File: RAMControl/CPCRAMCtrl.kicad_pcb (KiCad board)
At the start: 2 copper layers, 99.1 x 52.9 mm, 31 parts, among them IC112 74LS32, IC118 AMG40031, IC192 74LS32, J1 Conn_01x10_Female, J2 Conn_01x16_Female, U114 74LS373, U115 74LS244, U191 74LS04, U193 74LS08, U194 74LS173, U195 74LS74

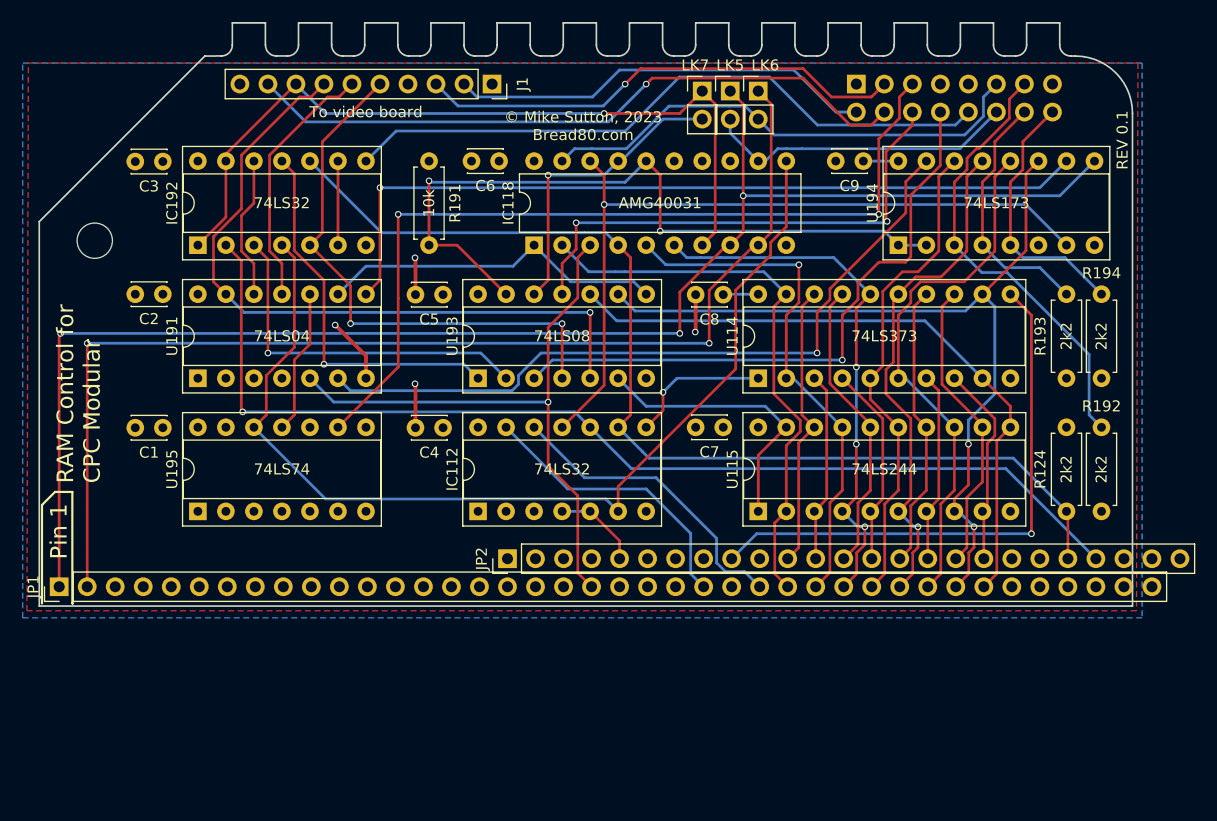
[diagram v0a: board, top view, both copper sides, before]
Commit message: Long overdue update...
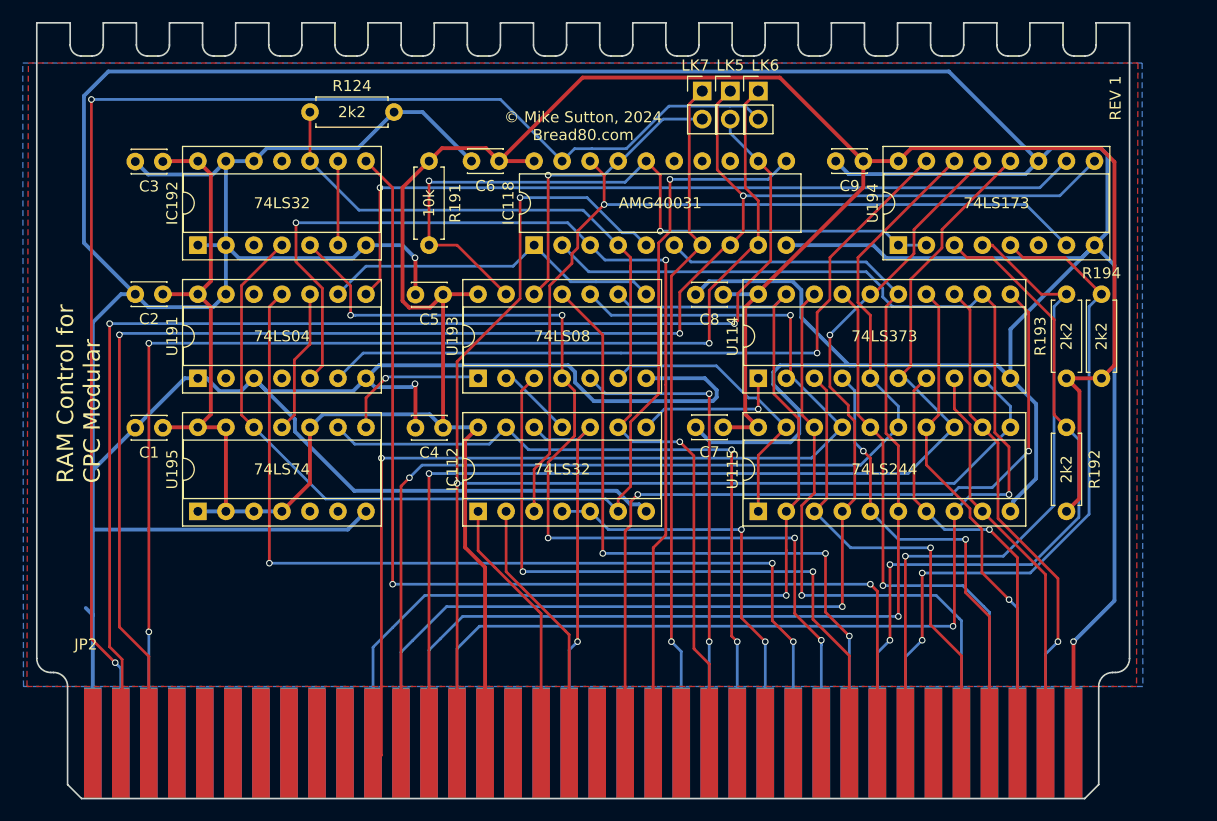
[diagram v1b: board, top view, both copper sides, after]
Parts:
- removed ?: , Mounting_Holes:MountingHole_3.2mm_M3
- removed J1: Conn_01x10_Female, Connector_PinSocket_2.54mm:PinSocket_1x10_P2.54mm_Vertical
- removed J2: Conn_01x16_Female, Connector_PinHeader_2.54mm:PinHeader_2x08_P2.54mm_Vertical
- JP1: value RC2014Bus -> CPCM_VideoRAM_EdgeBottom; footprint Connector_PinHeader_2.54mm:PinHeader_1x40_P2.54mm_Vertical -> CPCModular:Edge36_2.54PS; moved to B.Cu
- JP2: value RC2014ExtendedBus -> CPCM_VideoRAM_EdgeTop; footprint Connector_PinHeader_2.54mm:PinHeader_1x25_P2.54mm_Vertical -> CPCModular:Edge36_2.54PS
- moved R124 77.5 mm to (178.4, 108.6), turned to 0 degrees
- moved JP2 41.9 mm to (158.8, 167.6)
- moved JP1 12.7 mm to (158.8, 163.9), turned to 270 degrees
- moved R192 3.18 mm to (247.0, 144.8)
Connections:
- net ~CPU_ADDRx renamed /CRTC_ADDR_MULTI/~BUF_CPU_AD
- IC112 pad 1: GND -> /CRTC_ADDR_MULTI/~IORQ
- IC112 pad 12: /CRTC_ADDR_MULTI/~IORQ -> /~RAMRD
- IC112 pad 13: /CRTC_ADDR_MULTI/~WR -> /CRTC_ADDR_MULTI/~XCPU_AD
- IC112 pad 2: GND -> /CRTC_ADDR_MULTI/~WR
- IC118 pad 12: /CRTC_ADDR_MULTI/RAMA15 -> /CRTC_ADDR_MULTI/AOUT15
- IC118 pad 18: Net-(IC112-Pad11) -> Net-(IC112-Pad3)
- IC118 pad 19: /CRTC_ADDR_MULTI/RAMA14 -> /CRTC_ADDR_MULTI/AOUT14
- IC192 pad 1: /CRTC_ADDR_MULTI/~CAS -> GND
- IC192 pad 12: Net-(IC192-Pad12) -> GND
- IC192 pad 13: /CRTC_ADDR_MULTI/~CAS -> GND
- IC192 pad 2: /~RAMRD -> GND
- JP1 pad 1: A15 -> GND
- JP1 pad 11: Net-(JP1-Pad11) -> D6
- JP1 pad 12: Net-(JP1-Pad12) -> D4
- JP1 pad 13: Net-(JP1-Pad13) -> D2
- JP1 pad 14: Net-(JP1-Pad14) -> D0
- JP1 pad 17: GND -> Net-(JP1-Pad17)
- JP1 pad 18: +5V -> /~RAMRD
- JP1 pad 2: A14 -> /CRTC_ADDR_MULTI/AOUT14
- JP1 pad 20: /CRTC_ADDR_MULTI/~RESET -> Net-(JP1-Pad20)
- JP1 pad 22: Net-(JP1-Pad22) -> /CRTC_ADDR_MULTI/~CAS
- JP1 pad 23: Net-(JP1-Pad23) -> /CRTC_ADDR_MULTI/~244EN
- JP1 pad 24: /CRTC_ADDR_MULTI/~WR -> /CRTC_ADDR_MULTI/~XCPU_AD
- JP1 pad 25: Net-(JP1-Pad25) -> /~CPU_ADDR
- JP1 pad 26: /CRTC_ADDR_MULTI/~IORQ -> /CRTC_ADDR_MULTI/~RAS
- JP1 pad 27: D0 -> /CRTC_ADDR_MULTI/~MWE
- JP1 pad 28: D1 -> /CRTC_ADDR_MULTI/~RAMCS
- JP1 pad 29: D2 -> /CRTC_ADDR_MULTI/RAMA18
- JP1 pad 3: Net-(JP1-Pad3) -> A14
- JP1 pad 30: D3 -> /CRTC_ADDR_MULTI/RAMA16
- JP1 pad 31: D4 -> Net-(JP1-Pad31)
- JP1 pad 32: D5 -> RD6
- JP1 pad 33: D6 -> RD4
- JP1 pad 34: D7 -> RD2
- JP1 pad 35: Net-(JP1-Pad35) -> RD0
- JP2 pad 1: GND -> Net-(JP2-Pad1)
- JP2 pad 11: RAMD0 -> D7
- JP2 pad 12: RAMD1 -> D5
- JP2 pad 13: RAMD2 -> D3
- JP2 pad 14: RAMD3 -> D1
- JP2 pad 15: RAMD4 -> +5V
- JP2 pad 16: RAMD5 -> Net-(JP2-Pad16)
- JP2 pad 17: RAMD6 -> /CRTC_ADDR_MULTI/~IORQ
- JP2 pad 18: RAMD7 -> /CRTC_ADDR_MULTI/~WR
- JP2 pad 2: +5V -> /CRTC_ADDR_MULTI/AOUT15
- JP2 pad 20: Net-(JP2-Pad20) -> /READY
- JP2 pad 21: /RAMDIS -> /CRTC_ADDR_MULTI/~RESET
- JP2 pad 22: /~RAMRD -> Net-(JP2-Pad22)
- JP2 pad 23: Net-(JP2-Pad23) -> /RAMDIS
- JP2 pad 25: (no net) -> Net-(JP2-Pad25)
- JP2 pad 3: Net-(JP2-Pad3) -> A15
- JP2 pad 5: /~CPU_ADDR -> Net-(JP2-Pad5)
- JP2 pad 9: /READY -> Net-(JP2-Pad9)
- LK5 pad 2: /CRTC_ADDR_MULTI/RAMA15 -> /CRTC_ADDR_MULTI/AOUT15
- LK6 pad 2: /CRTC_ADDR_MULTI/RAMA14 -> /CRTC_ADDR_MULTI/AOUT14
- R192 pad 2: /CRTC_ADDR_MULTI/RAMA16 -> /CRTC_ADDR_MULTI/RAMA18
- R194 pad 2: /CRTC_ADDR_MULTI/RAMA18 -> /CRTC_ADDR_MULTI/RAMA16
- U114 pad 12: D6 -> D0
- U114 pad 13: RAMD6 -> RD0
- U114 pad 14: RAMD4 -> RD2
- U114 pad 15: D4 -> D2
- U114 pad 16: D2 -> D4
- U114 pad 17: RAMD2 -> RD4
- U114 pad 18: RAMD0 -> RD6
- U114 pad 19: D0 -> D6
- U114 pad 2: D1 -> D7
- U114 pad 3: RAMD1 -> RD7
- U114 pad 4: RAMD3 -> RD5
- U114 pad 5: D3 -> D5
- U114 pad 6: D5 -> D3
- U114 pad 7: RAMD5 -> RD3
- U114 pad 8: RAMD7 -> RD1
- U114 pad 9: D7 -> D1
- U115 pad 11: D7 -> D1
- U115 pad 12: RAMD6 -> RD0
- U115 pad 13: D5 -> D3
- U115 pad 14: RAMD4 -> RD2
- U115 pad 15: D3 -> D5
- U115 pad 16: RAMD2 -> RD4
- U115 pad 17: D1 -> D7
- U115 pad 18: RAMD0 -> RD6
- U115 pad 2: D0 -> D6
- U115 pad 3: RAMD1 -> RD7
- U115 pad 4: D2 -> D4
- U115 pad 5: RAMD3 -> RD5
- U115 pad 6: D4 -> D2
- U115 pad 7: RAMD5 -> RD3
- U115 pad 8: D6 -> D0
- U115 pad 9: RAMD7 -> RD1
- U191 pad 12: Net-(IC192-Pad12) -> Net-(U191-Pad12)
- U191 pad 13: /CRTC_ADDR_MULTI/~244EN -> GND
- U193 pad 1: Net-(IC192-Pad11) -> /CRTC_ADDR_MULTI/XCPU_AD
- U193 pad 2: Net-(IC192-Pad3) -> Net-(IC112-Pad11)
- U194 pad 11: D6 -> GND
- U194 pad 12: D5 -> D3
- U194 pad 14: D3 -> D5
- U194 pad 3: /CRTC_ADDR_MULTI/RAMA16 -> /CRTC_ADDR_MULTI/RAMA18
- U194 pad 5: /CRTC_ADDR_MULTI/RAMA18 -> /CRTC_ADDR_MULTI/RAMA16
- U194 pad 7: Net-(IC112-Pad11) -> Net-(IC112-Pad3)
- U195 pad 8: Net-(U195-Pad8) -> /CRTC_ADDR_MULTI/XCPU_AD
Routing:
- net GND: track 16.7 -> 586.4 mm, vias 4 -> 3
- net +5V: track 6.37 -> 288.7 mm
- net /CRTC_ADDR_MULTI/AOUT14: track 0.00 -> 124.7 mm, vias 0 -> 2
- net /CRTC_ADDR_MULTI/AOUT15: track 0.00 -> 116.7 mm, vias 0 -> 2
- net D0: track 51.6 -> 132.8 mm, vias 0 -> 2
- net Net-(IC112-Pad3): track 0.00 -> 78.3 mm, vias 0 -> 1
- net D1: track 47.7 -> 124.6 mm, vias 1 -> 2
- net /CRTC_ADDR_MULTI/~RAS: track 23.2 -> 89.4 mm, vias 0 -> 3
- net Net-(IC112-Pad11): track 69.7 -> 6.92 mm, vias 1 -> 0
- net D3: track 44.6 -> 106.5 mm, vias 0 -> 1
- net /~RAMRD: track 98.6 -> 37.3 mm
- net /~CCLK: track 61.2 -> 0.00 mm, vias 1 -> 0
- net D2: track 49.2 -> 106.4 mm, vias 3 -> 1
- net RD6: track 0.00 -> 57.1 mm, vias 0 -> 1
- net D5: track 48.6 -> 101.7 mm, vias 0 -> 1
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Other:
- board size 99.1 x 52.9 mm -> 99.1 x 70.3 mm
- board text added: "A modular Amstrad CPC compatible computer. All capacitors are 0.1uF/100nF. Other components as marked. Bread80.com - mstdn.social/@bread80 github.com/bread80"
- board text added: "REV 1"
- board text added: "© Mike Sutton, 2024 Bread80.com"
- board text removed: "A modular Amstrad CPC compatible using an RC2014 backplane. This is NOT an RC2014 module. All capacitors are 0.1uF/100nF. Other components as marked. Bread80.com - mstdn.social/@bread80 github.com/bread80 - twitter.com/bread80com"
- board text removed: "Pin 1"
- board text removed: "REV 0.1"
- board text removed: "To RAM board"
- board text removed: "To video board"
- board text removed: "© Mike Sutton, 2023 Bread80.com"
